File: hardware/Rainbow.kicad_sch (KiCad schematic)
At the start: 22 parts, among them J1 PICKit3, J2 UART, J3 BARREL_JACK, J4 HC-05, J5 RGB, Q1 Q_NMOS_GDS, Q2 Q_NMOS_GDS, Q3 Q_NMOS_GDS, SW1 SWITCH, U1 PIC16F15325, U2 MIC4574-5.0YN

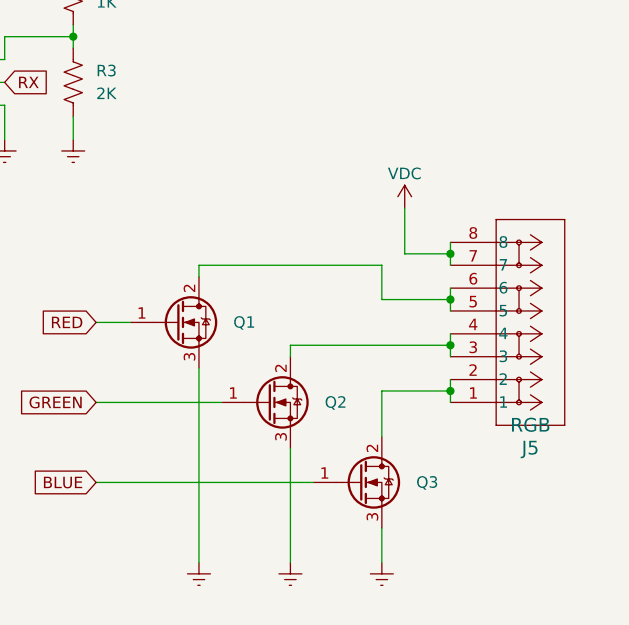
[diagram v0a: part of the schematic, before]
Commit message: Finish wiring
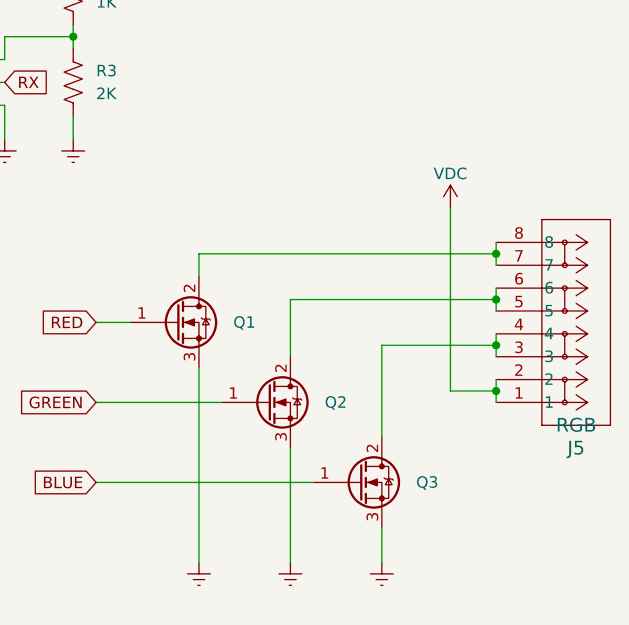
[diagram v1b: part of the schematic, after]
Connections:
- net VDC: now also J5.1, J5.2; no longer J5.7, J5.8
- net at J5.5, J5.6: now also Q2.2 (D); no longer Q1.2 (D)
- net at J5.3, J5.4: now also Q3.2 (D); no longer Q2.2 (D)
- new net: J5.7, J5.8, Q1.2 (D)
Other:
- moved on the sheet: J5
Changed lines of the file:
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@@
   (junction (at 101.6 138.43) (diameter 0) (color 0 0 0 0)
   )
+  (junction (at 189.23 82.55) (diameter 0) (color 0 0 0 0)
+  )
   (junction (at 162.56 140.97) (diameter 0) (color 0 0 0 0)
   )
@@
   (junction (at 142.24 58.42) (diameter 0) (color 0 0 0 0)
   )
+  (junction (at 189.23 97.79) (diameter 0) (color 0 0 0 0)
+  )
   (junction (at 177.8 140.97) (diameter 0) (color 0 0 0 0)
   )
@@
   (junction (at 177.8 135.89) (diameter 0) (color 0 0 0 0)
   )
-  (junction (at 184.15 82.55) (diameter 0) (color 0 0 0 0)
-  )
-  (junction (at 184.15 97.79) (diameter 0) (color 0 0 0 0)
-  )
-  (junction (at 184.15 87.63) (diameter 0) (color 0 0 0 0)
+  (junction (at 189.23 87.63) (diameter 0) (color 0 0 0 0)
+  )
+  (junction (at 189.23 92.71) (diameter 0) (color 0 0 0 0)
   )
   (junction (at 82.55 143.51) (diameter 0) (color 0 0 0 0)
-  )
-  (junction (at 184.15 92.71) (diameter 0) (color 0 0 0 0)
   )
   (no_connect (at 67.31 101.6))
@@
     (stroke (width 0) (type default) (color 0 0 0 0))
   )
-  (wire (pts (xy 184.15 96.52) (xy 184.15 97.79))
-    (stroke (width 0) (type default) (color 0 0 0 0))
-  )
-  (wire (pts (xy 176.53 97.79) (xy 184.15 97.79))
+  (wire (pts (xy 189.23 96.52) (xy 189.23 97.79))
     (stroke (width 0) (type default) (color 0 0 0 0))
   )
@@
     (stroke (width 0) (type default) (color 0 0 0 0))
   )
+  (wire (pts (xy 189.23 97.79) (xy 189.23 99.06))
+    (stroke (width 0) (type default) (color 0 0 0 0))
+  )
   (wire (pts (xy 129.54 135.89) (xy 129.54 137.16))
     (stroke (width 0) (type default) (color 0 0 0 0))
@@
     (stroke (width 0) (type default) (color 0 0 0 0))
   )
-  (wire (pts (xy 184.15 82.55) (xy 184.15 83.82))
+  (wire (pts (xy 189.23 81.28) (xy 189.23 82.55))
     (stroke (width 0) (type default) (color 0 0 0 0))
   )
@@
     (stroke (width 0) (type default) (color 0 0 0 0))
   )
-  (wire (pts (xy 184.15 92.71) (xy 184.15 93.98))
+  (wire (pts (xy 189.23 91.44) (xy 189.23 92.71))
     (stroke (width 0) (type default) (color 0 0 0 0))
   )
@@
     (stroke (width 0) (type default) (color 0 0 0 0))
   )
-  (wire (pts (xy 179.07 77.47) (xy 179.07 82.55))
+  (wire (pts (xy 184.15 77.47) (xy 184.15 97.79))
+    (stroke (width 0) (type default) (color 0 0 0 0))
+  )
+  (wire (pts (xy 184.15 97.79) (xy 189.23 97.79))
     (stroke (width 0) (type default) (color 0 0 0 0))
   )
@@
     (stroke (width 0) (type default) (color 0 0 0 0))
   )
-  (wire (pts (xy 166.37 93.98) (xy 166.37 92.71))
-    (stroke (width 0) (type default) (color 0 0 0 0))
-  )
   (wire (pts (xy 134.62 66.04) (xy 134.62 69.85))
     (stroke (width 0) (type default) (color 0 0 0 0))
   )
-  (wire (pts (xy 156.21 85.09) (xy 156.21 83.82))
+  (wire (pts (xy 156.21 82.55) (xy 156.21 85.09))
     (stroke (width 0) (type default) (color 0 0 0 0))
   )
@@
     (stroke (width 0) (type default) (color 0 0 0 0))
   )
+  (wire (pts (xy 189.23 87.63) (xy 189.23 88.9))
+    (stroke (width 0) (type default) (color 0 0 0 0))
+  )
+  (wire (pts (xy 166.37 87.63) (xy 166.37 93.98))
+    (stroke (width 0) (type default) (color 0 0 0 0))
+  )
   (wire (pts (xy 134.62 58.42) (xy 142.24 58.42))
     (stroke (width 0) (type default) (color 0 0 0 0))
@@
     (stroke (width 0) (type default) (color 0 0 0 0))
   )
-  (wire (pts (xy 156.21 83.82) (xy 176.53 83.82))
-    (stroke (width 0) (type default) (color 0 0 0 0))
-  )
   (wire (pts (xy 101.6 144.78) (xy 101.6 138.43))
     (stroke (width 0) (type default) (color 0 0 0 0))
@@
     (stroke (width 0) (type default) (color 0 0 0 0))
   )
-  (wire (pts (xy 184.15 97.79) (xy 184.15 99.06))
-    (stroke (width 0) (type default) (color 0 0 0 0))
-  )
-  (wire (pts (xy 176.53 83.82) (xy 176.53 87.63))
-    (stroke (width 0) (type default) (color 0 0 0 0))
-  )
   (wire (pts (xy 176.53 113.03) (xy 176.53 116.84))
     (stroke (width 0) (type default) (color 0 0 0 0))
@@
     (stroke (width 0) (type default) (color 0 0 0 0))
   )
+  (wire (pts (xy 176.53 92.71) (xy 189.23 92.71))
+    (stroke (width 0) (type default) (color 0 0 0 0))
+  )
   (wire (pts (xy 144.78 107.95) (xy 168.91 107.95))
     (stroke (width 0) (type default) (color 0 0 0 0))
@@
     (stroke (width 0) (type default) (color 0 0 0 0))
   )
-  (wire (pts (xy 179.07 82.55) (xy 184.15 82.55))
-    (stroke (width 0) (type default) (color 0 0 0 0))
-  )
   (wire (pts (xy 134.62 60.96) (xy 134.62 58.42))
     (stroke (width 0) (type default) (color 0 0 0 0))
@@
     (stroke (width 0) (type default) (color 0 0 0 0))
   )
-  (wire (pts (xy 184.15 86.36) (xy 184.15 87.63))
+  (wire (pts (xy 189.23 86.36) (xy 189.23 87.63))
     (stroke (width 0) (type default) (color 0 0 0 0))
   )
@@
     (stroke (width 0) (type default) (color 0 0 0 0))
   )
+  (wire (pts (xy 189.23 82.55) (xy 189.23 83.82))
+    (stroke (width 0) (type default) (color 0 0 0 0))
+  )
   (wire (pts (xy 115.57 109.22) (xy 115.57 115.57))
     (stroke (width 0) (type default) (color 0 0 0 0))
@@
     (stroke (width 0) (type default) (color 0 0 0 0))
   )
-  (wire (pts (xy 176.53 102.87) (xy 176.53 97.79))
+  (wire (pts (xy 176.53 92.71) (xy 176.53 102.87))
     (stroke (width 0) (type default) (color 0 0 0 0))
   )
@@
     (stroke (width 0) (type default) (color 0 0 0 0))
   )
-  (wire (pts (xy 176.53 87.63) (xy 184.15 87.63))
-    (stroke (width 0) (type default) (color 0 0 0 0))
-  )
   (wire (pts (xy 77.47 63.5) (xy 77.47 72.39))
     (stroke (width 0) (type default) (color 0 0 0 0))
@@
     (stroke (width 0) (type default) (color 0 0 0 0))
   )
+  (wire (pts (xy 156.21 82.55) (xy 189.23 82.55))
+    (stroke (width 0) (type default) (color 0 0 0 0))
+  )
   (wire (pts (xy 57.15 104.14) (xy 67.31 104.14))
     (stroke (width 0) (type default) (color 0 0 0 0))
   )
-  (wire (pts (xy 184.15 81.28) (xy 184.15 82.55))
-    (stroke (width 0) (type default) (color 0 0 0 0))
-  )
-  (wire (pts (xy 184.15 91.44) (xy 184.15 92.71))
+  (wire (pts (xy 189.23 92.71) (xy 189.23 93.98))
     (stroke (width 0) (type default) (color 0 0 0 0))
   )
@@
     (stroke (width 0) (type default) (color 0 0 0 0))
   )
-  (wire (pts (xy 166.37 92.71) (xy 184.15 92.71))
-    (stroke (width 0) (type default) (color 0 0 0 0))
-  )
   (wire (pts (xy 115.57 82.55) (xy 115.57 86.36))
     (stroke (width 0) (type default) (color 0 0 0 0))
@@
     (stroke (width 0) (type default) (color 0 0 0 0))
   )
-  (wire (pts (xy 184.15 87.63) (xy 184.15 88.9))
+  (wire (pts (xy 166.37 87.63) (xy 189.23 87.63))
     (stroke (width 0) (type default) (color 0 0 0 0))
   )
@@
     (pin "6")
   )
-  (symbol (lib_id "Rainbow:Wago") (at 194.31 88.9 0) (mirror x) (unit 1)
+  (symbol (lib_id "Rainbow:Wago") (at 199.39 88.9 0) (mirror x) (unit 1)
     (in_bom yes) (on_board yes)
-    (property "Reference" "J5" (id 0) (at 193.04 104.14 0)
+    (property "Reference" "J5" (id 0) (at 198.12 104.14 0)
       (effects (font (size 1.524 1.524)))
     )
-    (property "Value" "RGB" (id 1) (at 193.04 101.6 0)
+    (property "Value" "RGB" (id 1) (at 198.12 101.6 0)
       (effects (font (size 1.524 1.524)))
     )
-    (property "Footprint" "Rainbow:Wago" (id 2) (at 194.31 88.9 0)
+    (property "Footprint" "Rainbow:Wago" (id 2) (at 199.39 88.9 0)
       (effects (font (size 1.27 1.27) italic) hide)
     )
-    (property "Datasheet" "" (id 3) (at 194.31 88.9 0)
+    (property "Datasheet" "" (id 3) (at 199.39 88.9 0)
       (effects (font (size 1.27 1.27) italic) hide)
     )
@@
     (pin "1")
   )
-  (symbol (lib_id "power:VDC") (at 179.07 77.47 0) (unit 1)
+  (symbol (lib_id "power:VDC") (at 184.15 77.47 0) (unit 1)
     (in_bom yes) (on_board yes)
-    (property "Reference" "#PWR014" (id 0) (at 179.07 80.01 0)
-      (effects (font (size 1.27 1.27)) hide)
-    )
-    (property "Value" "VDC" (id 1) (at 179.07 73.66 0))
-    (property "Footprint" "" (id 2) (at 179.07 77.47 0)
-      (effects (font (size 1.27 1.27)) hide)
-    )
-    (property "Datasheet" "" (id 3) (at 179.07 77.47 0)
-      (effects (font (size 1.27 1.27)) hide)
-    )
+    (property "Reference" "#PWR014" (id 0) (at 184.15 80.01 0)
+      (effects (font (size 1.27 1.27)) hide)
+    )
+    (property "Value" "VDC" (id 1) (at 184.15 73.66 0))
+    (property "Footprint" "" (id 2) (at 184.15 77.47 0)
+      (effects (font (size 1.27 1.27)) hide)
+    )
+    (property "Datasheet" "" (id 3) (at 184.15 77.47 0)
+      (effects (font (size 1.27 1.27)) hide)
+    )
